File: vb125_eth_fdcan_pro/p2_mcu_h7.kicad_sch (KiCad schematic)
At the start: 63 parts, among them J1 MEM2061-01-188-00-A, J2 TAGconnect NL, J3 Conn_02x20_Pin, M1 DM-OLED042-647, SW1 KSS331GLFS, U1 STM32H725IGKx, X1 ECX-.327-CDX-1293

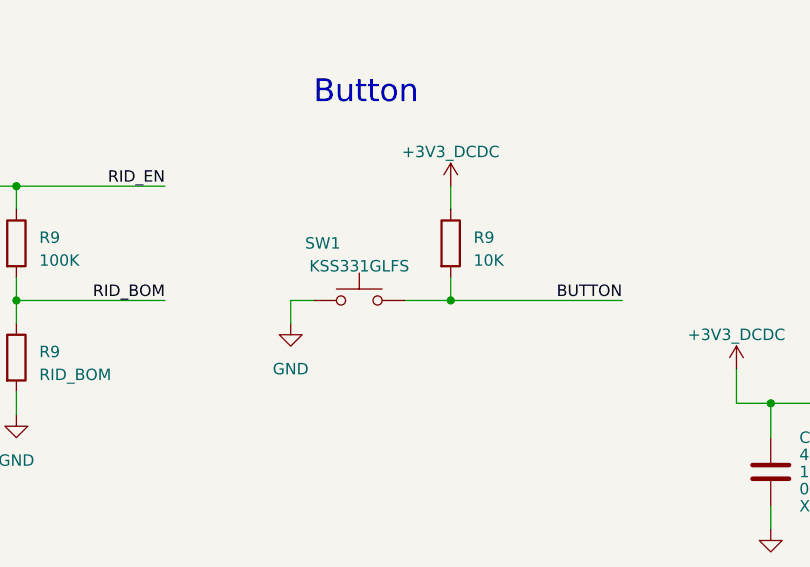
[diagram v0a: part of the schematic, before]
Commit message: Continue with floorplan
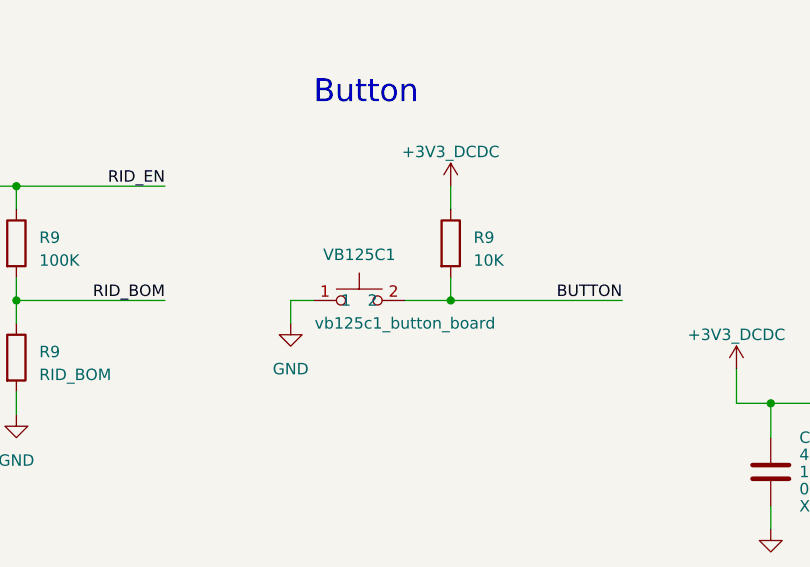
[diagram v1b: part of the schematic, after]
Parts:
- removed SW1: KSS331GLFS, vhrd_electromechanical:SW_KSS3, symbol Switch:SW_Push
- added VB125C1: vb125c1_button_board, vhrd_boards:vb125c1_button_board, symbol vhrd_boards:vb125c1_button_board
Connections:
- net BUTTON: now also VB125C1.2
- net GND: now also VB125C1.1
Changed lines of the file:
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@@
-    )
-  )
-  (symbol (lib_id "Switch:SW_Push") (at 154.94 180.34 0) (unit 1)
-    (in_bom yes) (on_board yes) (dnp no) (fields_autoplaced)
-    (property "Reference" "SW1" (at 148.9117 173.99 0)
-      (effects (font (size 1.27 1.27)) (justify left))
-    )
-    (property "Value" "KSS331GLFS" (at 154.94 176.53 0)
-      (effects (font (size 1.27 1.27)))
-    )
-    (property "Footprint" "vhrd_electromechanical:SW_KSS3" (at 154.94 175.26 0)
-      (effects (font (size 1.27 1.27)) hide)
-    )
-    (property "Datasheet" "~" (at 154.94 175.26 0)
-      (effects (font (size 1.27 1.27)) hide)
-    )
-    (pin "1")
-    (pin "2")
-    (instances
-      (project "vb125_eth_fdcan_pro"
-        (path "/b473bccb-f14c-41d5-b473-137d3ef8ae1e/c16e79c7-955f-4686-8fe9-acff02e57751"
-          (reference "SW1") (unit 1)
-        )
-      )
     )
   )
@@
         )
       )
+    )
+  )
+  (symbol (lib_id "vhrd_boards:vb125c1_button_board") (at 154.94 180.34 0) (unit 1)
+    (in_bom yes) (on_board yes) (dnp no)
+    (property "Reference" "VB125C1" (at 154.94 175.26 0)
+      (effects (font (size 1.27 1.27)))
+    )
+    (property "Value" "vb125c1_button_board" (at 160.02 182.88 0)
+      (effects (font (size 1.27 1.27)))
+    )
+    (property "Footprint" "vhrd_boards:vb125c1_button_board" (at 154.94 182.88 0)
+      (effects (font (size 1.27 1.27)) hide)
+    )
+    (property "Datasheet" "" (at 154.94 180.34 0)
+      (effects (font (size 1.27 1.27)) hide)
+    )
+    (pin "1")
+    (pin "2")
+    (instances
+      (project "vb125_eth_fdcan_pro"
+        (path "/b473bccb-f14c-41d5-b473-137d3ef8ae1e/c16e79c7-955f-4686-8fe9-acff02e57751"
+          (reference "VB125C1") (unit 1)
+        )
+      )
